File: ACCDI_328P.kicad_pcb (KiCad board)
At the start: 2 copper layers, 150.1 x 82.2 mm, 44 parts, among them IC1 MJE340G, J1 Conn_01x05_Female, Q1 2N2222, Q2 2N2222, U1 LR8N3-G, U2 ATmega328P-P, Y1 16Mhz

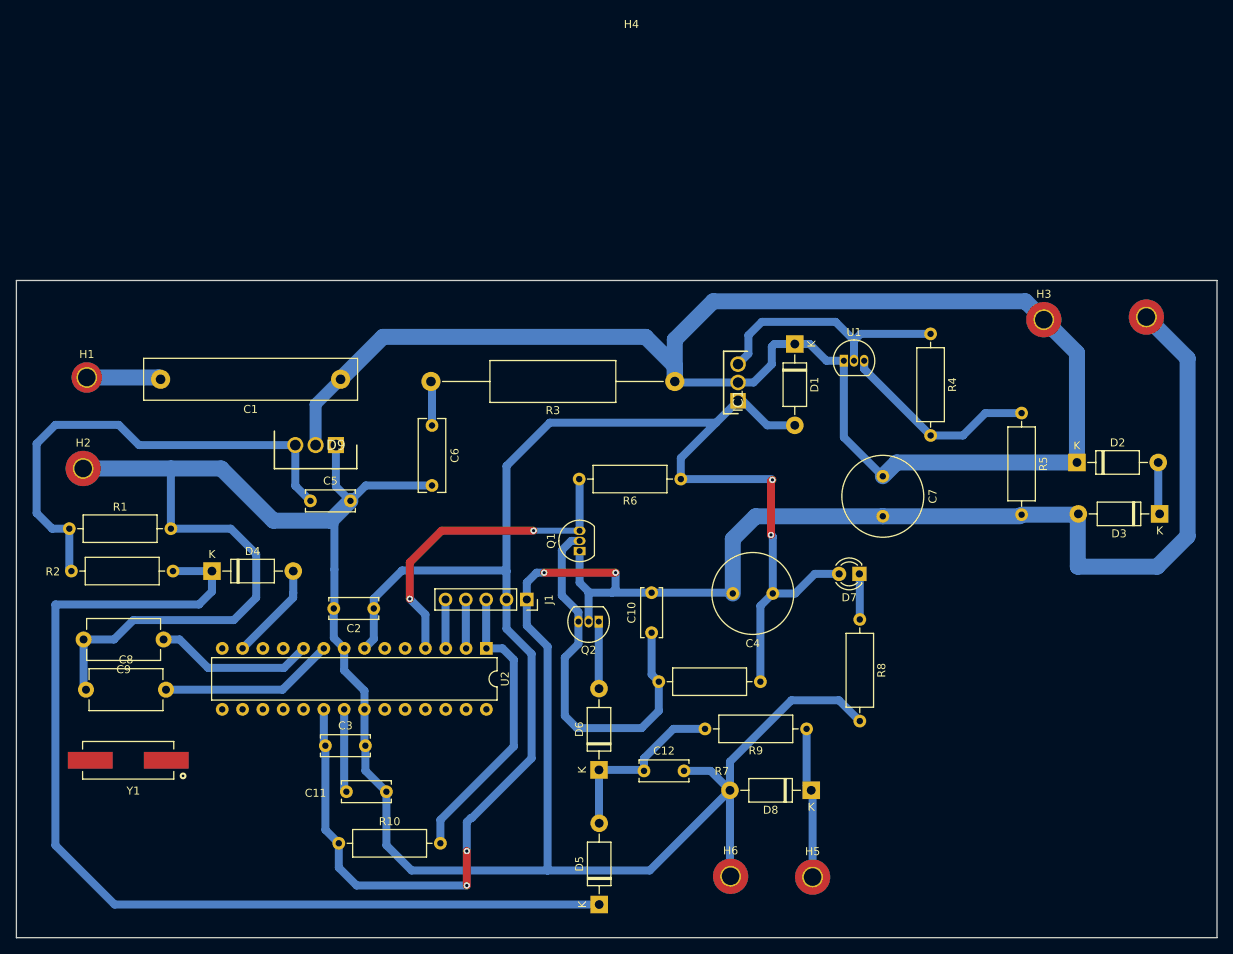
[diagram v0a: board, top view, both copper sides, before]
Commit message: 2 layer board
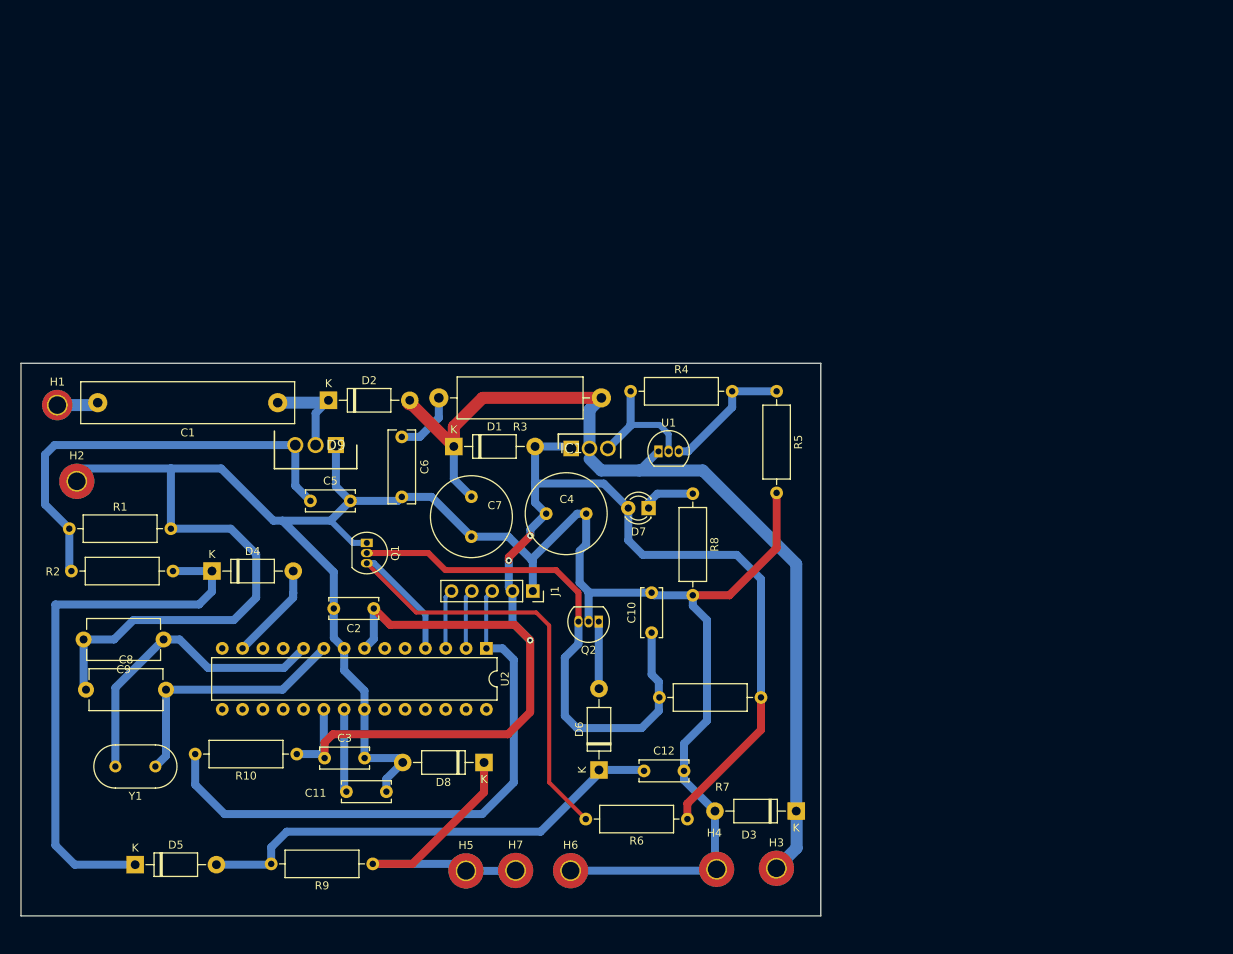
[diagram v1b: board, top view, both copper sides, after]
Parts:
- added H7: Kill Switch, MountingHole:MountingHole_2.2mm_M2_Pad_TopBottom, F.Cu at (138.3, 115.9)
- R3: footprint Resistor_THT:R_Axial_DIN0516_L15.5mm_D5.0mm_P30.48mm_Horizontal -> Resistor_THT:R_Axial_DIN0516_L15.5mm_D5.0mm_P20.32mm_Horizontal
- Y1: value 16Mhz -> HC49S-16-30-50-70-30-ATF; footprint ABLS2-12:XTAL_ABLS2-12.000MHZ-B1U-T -> Crystal:Resonator-2Pin_W10.0mm_H5.0mm
- moved D2 93.9 mm to (114.9, 57.1)
- moved H4 87.5 mm to (163.4, 115.8)
- moved H3 76.3 mm to (170.9, 115.7)
- moved D3 58.7 mm to (173.4, 108.5)
- moved D5 58.2 mm to (90.8, 115.2), turned to 0 degrees
- moved R9 56.8 mm to (120.5, 115.1)
- moved C7 51.5 mm to (132.8, 69.2)
- moved D1 44.5 mm to (130.6, 62.9), turned to 0 degrees
- moved H5 43.3 mm to (132.1, 116.0)
- moved R6 42.5 mm to (159.8, 109.5)
- moved D8 41.0 mm to (134.4, 102.4)
- moved R4 38.2 mm to (152.7, 56.0), turned to 0 degrees
- moved R5 30.7 mm to (170.9, 56.0)
- moved C4 30.0 mm to (142.2, 71.3), turned to 0 degrees
- moved D7 27.6 mm to (154.9, 70.6)
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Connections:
- IC1 pad 3: Souce_coil -> Net-(IC1-Pad3)
- R4 pad 1: Souce_coil -> Net-(IC1-Pad3)
- U1 pad 2: Souce_coil -> Net-(IC1-Pad3)
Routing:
- net GND: track 425.9 -> 292.3 mm, vias 2 -> 0
- net Souce_coil: track 235.8 -> 132.4 mm
- net SCR_gate: track 128.8 -> 68.7 mm
- net +5 Volt: track 215.8 -> 176.5 mm, vias 5 -> 3
- net Net-(C12-Pad1): track 23.1 -> 59.9 mm
- net Net-(J1-Pad3): track 36.9 -> 73.7 mm
- net Pickup_circuit: track 40.9 -> 66.3 mm, vias 2 -> 0
- net Net-(D8-Pad1): track 18.8 -> 40.8 mm
- net Net-(C10-Pad1): track 48.4 -> 68.0 mm
- net Net-(C9-Pad1): track 20.0 -> 38.3 mm
- net Net-(IC1-Pad3): track 0.00 -> 15.7 mm
- net Net-(C8-Pad2): track 21.9 -> 32.0 mm
- net Net-(R4-Pad2): track 25.3 -> 16.5 mm
- net Net-(C5-Pad1): track 61.1 -> 55.5 mm
- net Net-(C1-Pad2): track 9.32 -> 5.17 mm
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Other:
- board size 150.1 x 82.2 mm -> 100 x 69.1 mm
